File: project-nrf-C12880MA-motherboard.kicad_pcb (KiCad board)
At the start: 2 copper layers, 86.4 x 57.1 mm, 26 parts, among them J1 Left, J2 Right, J3 PJ-036AH-SMT-TR, J4 SM04B-SRSS-TB(LF)(SN), J5 SM04B-SRSS-TB(LF)(SN), J6 SM04B-SRSS-TB(LF)(SN), J7 1702473, J8 C12880MA Breakboard v2, U1 ADS1219IPWR, U2 TPS7A0350PDBVR, U3 LSF0204DPWR

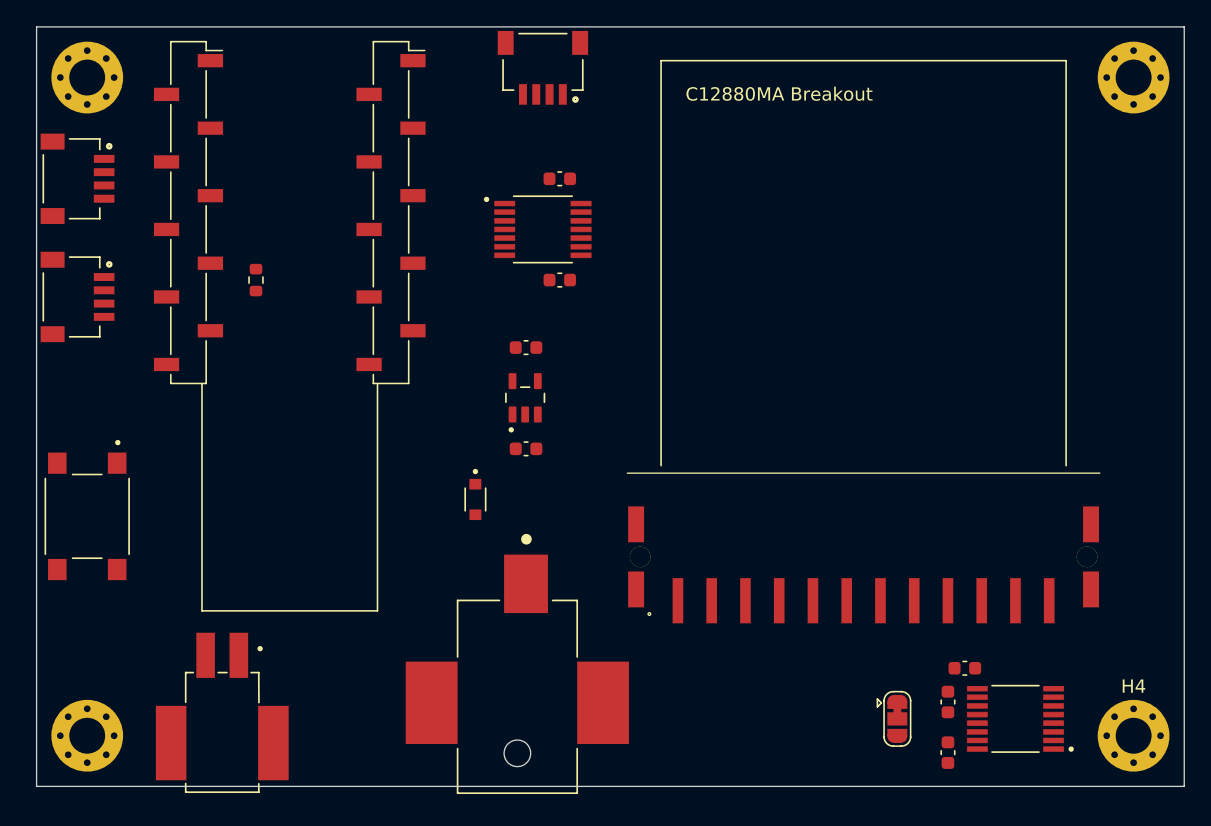
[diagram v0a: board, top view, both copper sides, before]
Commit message: Placement 2
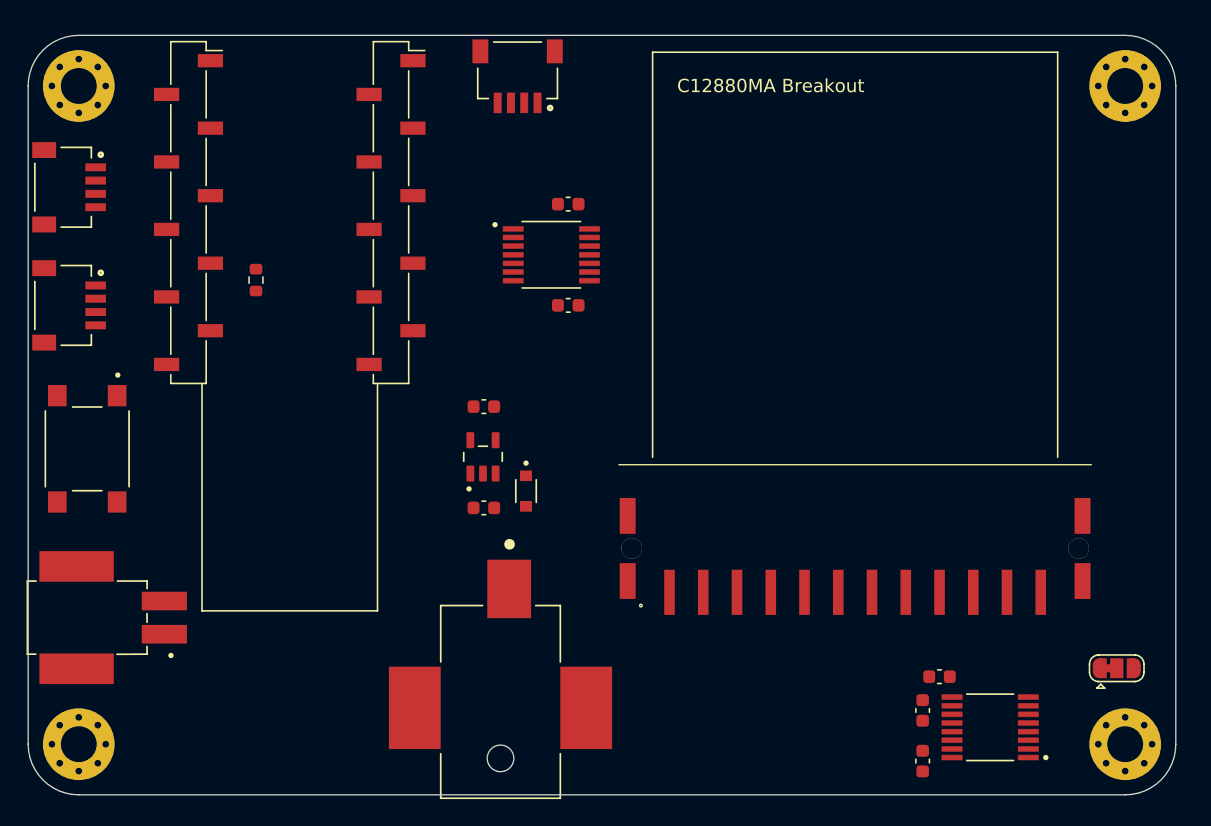
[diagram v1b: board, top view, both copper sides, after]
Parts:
- moved JP1 16.9 mm to (96.5, 68.6), turned to 0 degrees
- moved J7 13.3 mm to (19.1, 64.8), turned to 270 degrees
- moved C2 5.46 mm to (48.9, 56.5)
- moved C3 5.46 mm to (48.9, 48.9)
- moved U2 5.46 mm to (48.8, 52.7)
- moved S1 5.08 mm to (19.1, 52.1)
- moved D1 3.86 mm to (52.1, 55.2)
- moved C1 2.01 mm to (83.2, 69.2)
- moved U1 2.01 mm to (87.0, 73.0)
- moved J6 2.01 mm to (51.4, 26.0)
- moved C6 2.01 mm to (55.2, 41.3)
- moved C7 2.01 mm to (55.2, 33.7)
- moved U3 2.01 mm to (54.0, 37.5)
- moved C4 2.01 mm to (81.9, 71.8)
- moved C5 2.01 mm to (81.9, 75.6)
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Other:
- board size 86.4 x 57.1 mm -> 86.4 x 57.2 mm
